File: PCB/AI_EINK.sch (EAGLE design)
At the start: 188 parts, among them IC3 WM8960, J1 BM04B-GHS-TBT(LF)(SN)(N), J2 C393939, J3 524372471, Q1 SI1308EDL-T1-GE3, Q3 NMOS_C7465427, T1 MMUN2133LT1G, U1 TPS61092RSAR, U10 AP2112-3.3K, U11 AP2112-3.3K, U12 SPU0410LR5H-QB, U2 MC74VHC1G14DFT1G, U3 BQ27441DRZR-G1A, U4 BQ24075, U5 TLV74328, U6 TLV74315, U7 TLV74318PDBVRDBV0005A_L, U8 ST25DV64K-IER6S3SOIC_IER6S3_S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, U9 EMC2301-1-ACZL-TRMSOP8_MC_MCH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, Y1 ABM8-272-T3

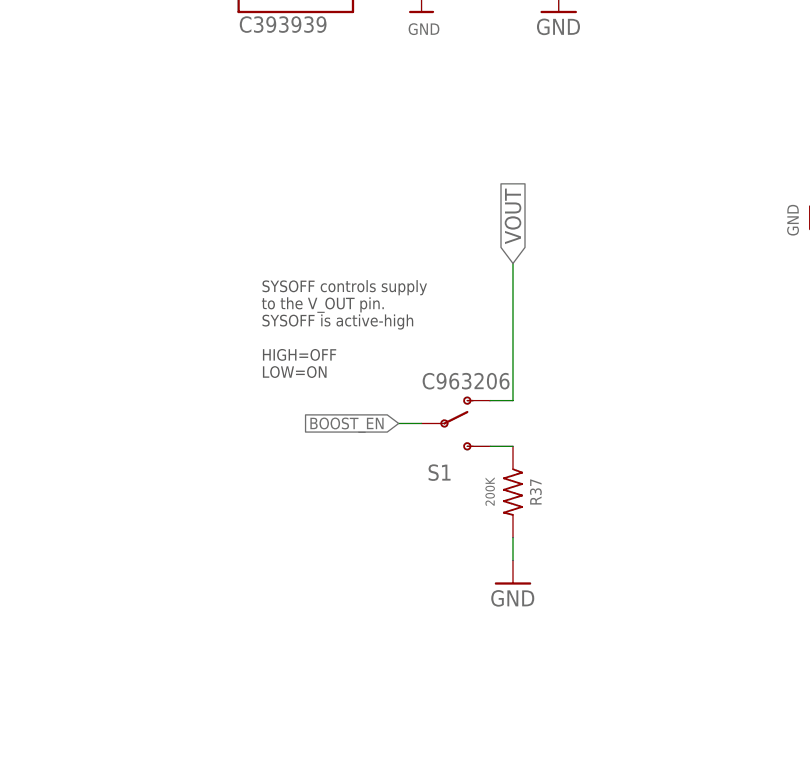
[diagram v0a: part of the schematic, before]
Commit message: kevin commit
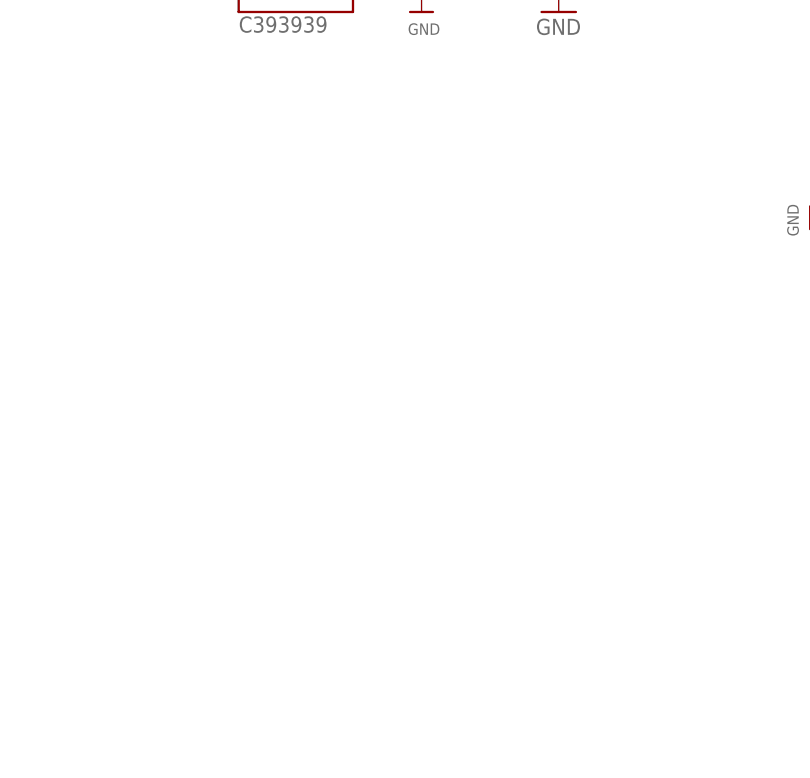
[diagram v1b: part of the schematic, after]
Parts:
- removed R37: 200K, resistor:R-US_R0603
- removed S1: C963206, SparkFun-Electromechanical:SWITCH-SPDT-SMD-A
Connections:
- removed net N$27: R37.1, S1.S
- net BOOST_EN: no longer S1.P
- net GND: no longer R37.2
- net VOUT: no longer S1.O
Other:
- note removed: "SYSOFF controls supply to the V_OUT pin. SYSOFF is active-high HIGH=OFF LOW=ON"
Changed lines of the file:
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@@
 <attribute name="PROD_ID" value="RES-13217"/>
 </part>
-<part name="GND18" library="SparkFun-Aesthetics" deviceset="GND" device=""/>
-<part name="S1" library="SparkFun-Electromechanical" deviceset="SWITCH-SPDT" device="-SMD-A" value="C963206"/>
 <part name="R7" library="resistor" library_urn="urn:adsk.eagle:library:348" deviceset="R-US_" device="R0603" package3d_urn="urn:adsk.eagle:package:23555/3" value="1.1k">
 <attribute name="PROD_ID" value="RES-10447"/>
@@
 <part name="GND35" library="SparkFun-Aesthetics" deviceset="GND" device=""/>
 <part name="R36" library="resistor" library_urn="urn:adsk.eagle:library:348" deviceset="R-US_" device="R0603" package3d_urn="urn:adsk.eagle:package:23555/3" value="200K"/>
-<part name="R37" library="resistor" library_urn="urn:adsk.eagle:library:348" deviceset="R-US_" device="R0603" package3d_urn="urn:adsk.eagle:package:23555/3" value="200K"/>
 <part name="R28" library="resistor" library_urn="urn:adsk.eagle:library:348" deviceset="R-US_" device="R0603" package3d_urn="urn:adsk.eagle:package:23555/3" value="10k"/>
 <part name="GND28" library="supply1" library_urn="urn:adsk.eagle:library:371" deviceset="GND" device=""/>
@@
      (Good IN supply)
   - Open (LED disconnected)</text>
-<text x="637.54" y="180.34" size="1.27" layer="97" font="vector">SYSOFF controls supply
-to the V_OUT pin.
-SYSOFF is active-high
-HIGH=OFF
-LOW=ON</text>
 <text x="492.76" y="106.68" size="2.54" layer="94" font="vector" align="top-left">EINK HiGH VOLTAGE MODULE</text>
 <text x="505.46" y="294.64" size="2.54" layer="94" font="vector" align="top-left">5V BOOST</text>
@@
 <attribute name="PROD_ID" x="307.34" y="226.06" size="1.524" layer="96" rot="R270" align="top-left" display="off"/>
 </instance>
-<instance part="GND18" gate="1" x="665.48" y="157.48" smashed="yes">
-<attribute name="VALUE" x="662.94" y="154.94" size="1.778" layer="96"/>
-</instance>
-<instance part="S1" gate="1" x="657.86" y="175.26" smashed="yes">
-<attribute name="NAME" x="655.955" y="168.91" size="1.778" layer="95"/>
-<attribute name="VALUE" x="655.32" y="179.07" size="1.778" layer="96"/>
-</instance>
 <instance part="R7" gate="G$1" x="322.58" y="223.52" smashed="yes" rot="R270">
 <attribute name="NAME" x="324.0786" y="227.33" size="1.778" layer="95" font="vector" rot="R270"/>
@@
 <attribute name="VALUE" x="822.96" y="198.12" size="1.016" layer="96" font="vector" ratio="15" rot="R270" align="center"/>
 </instance>
-<instance part="R37" gate="G$1" x="665.48" y="167.64" smashed="yes" rot="R270">
-<attribute name="NAME" x="668.02" y="167.64" size="1.27" layer="95" font="vector" rot="R270" align="center"/>
-<attribute name="VALUE" x="662.94" y="167.64" size="1.016" layer="96" font="vector" ratio="15" rot="R270" align="center"/>
-</instance>
 <instance part="R28" gate="G$1" x="690.88" y="76.2" smashed="yes">
 <attribute name="NAME" x="687.07" y="77.6986" size="1.778" layer="95"/>
@@
 </segment>
 <segment>
-<pinref part="GND18" gate="1" pin="GND"/>
-<pinref part="R37" gate="G$1" pin="2"/>
-<wire x1="665.48" y1="160.02" x2="665.48" y2="162.56" width="0.1524" layer="91"/>
-</segment>
-<segment>
 <pinref part="R28" gate="G$1" pin="1"/>
 <wire x1="685.8" y1="76.2" x2="680.72" y2="76.2" width="0.1524" layer="91"/>
@@
 <net name="BOOST_EN" class="0">
 <segment>
-<wire x1="655.32" y1="175.26" x2="652.78" y2="175.26" width="0.1524" layer="91"/>
-<label x="652.78" y="175.26" size="1.27" layer="95" font="vector" rot="R180" xref="yes"/>
-<pinref part="S1" gate="1" pin="P"/>
-</segment>
-<segment>
 <pinref part="R13" gate="G$1" pin="1"/>
 <wire x1="533.4" y1="274.32" x2="533.4" y2="276.86" width="0.1524" layer="91"/>
@@
 <pinref part="R36" gate="G$1" pin="1"/>
 </segment>
-<segment>
-<label x="665.48" y="193.04" size="1.778" layer="95" rot="R90" xref="yes"/>
-<wire x1="662.94" y1="177.8" x2="665.48" y2="177.8" width="0.1524" layer="91"/>
-<pinref part="S1" gate="1" pin="O"/>
-<wire x1="665.48" y1="177.8" x2="665.48" y2="193.04" width="0.1524" layer="91"/>
-</segment>
 </net>
 <net name="N$7" class="0">
@@
 </segment>
 </net>
-<net name="N$27" class="0">
-<segment>
-<pinref part="R37" gate="G$1" pin="1"/>
-<pinref part="S1" gate="1" pin="S"/>
-<wire x1="665.48" y1="172.72" x2="662.94" y2="172.72" width="0.1524" layer="91"/>
-</segment>
-</net>

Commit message: PCB V3
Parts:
- removed ANT1: NFC_ANTENNA_25X15, microbuilder:NFC_ANTENNA_25X15
- removed C25, C30: 1.0uF, Capacitor:C_CHIP-0603(1608-METRIC)
- removed C27, C70, C78, C81: 0.1uF, Capacitor:C_CHIP-0603(1608-METRIC)
- removed C28, C29, C31, C32, C33, C34, C35, C36, C37, C38, C39, C41, C51: 10uF, Capacitor:C_CHIP-0603(1608-METRIC)
- removed FB10, FB9: 120o, microbuilder:FERRITE-0805NO
- removed FL3, FL4, FL5: BLM18HE152SN1D, BLM18HE152SN1D:BLM18HE152SN1D
- removed GND25, RPIBOOT3: DNP, SparkFun-Connectors:TEST-POINT3
- removed OSC1: 24MHz 3.3V Oscillator, microbuilder:OSCILLATOR3.2X2.5
- removed OV5674: DF30FC-24DS-0.4V(82)CONN_DF30FC-24DS-0.4V(82)_HIR, 2024-03-07_05-07-01_Library:DF30FC-24DS-0.4V(82)CONN_DF30FC-24DS-0.4V(82)_HIR
- removed SJ2, SJ3: DNP, SparkFun-Passives:JUMPER-PAD-3-2OF3_NC_BY_TRACE_SMALL
- removed SPI_FLASH_SAM: W25Q128JVBIQTFBGA_128JVBIQ_WIN, 2024-03-10_02-04-46_Library:W25Q128JVBIQTFBGA_128JVBIQ_WIN
- removed U$10, U$11, U$94, U$95: MOUNTINGHOLE2.5, microbuilder:MOUNTINGHOLE2.5
- removed U7: TLV74318PDBVRDBV0005A_L, 2024-03-10_03-34-55_Library:TLV74318PDBVRDBV0005A_L
- added CAMERA: 524372271CON_524372271_MOL, 2024-03-29_02-21-27_Library:524372271CON_524372271_MOL
- added FB1, FB4: FERRITE_BEAD, Filter:FBCHIP-0603(1608-METRIC)
- added JOY_STICK: BM04B-GHS-TBT(LF)(SN)(N), BM04B-GHS-TBT_LF__SN__N_:BM04B-GHS-TBT(LF)(SN)(N)
- added M.2KEYM(NGFF): 1-2199119-5, 1-2199119-5:1-2199119-5
- added Q2: NMOS_C7465427, Transistor:NMOSFETSOT23-GSD
- added R19: 5.1K, Resistor:R-US_CHIP-0402(1005-METRIC)
- added R21: 5.1k, Resistor:R-US_CHIP-0402(1005-METRIC)
- added R25, R26: 4.7K, Resistor:R-US_CHIP-0402(1005-METRIC)
- added U13: TPD4EUSB30DQARDQA10, 2024-03-29_01-35-38_Library:TPD4EUSB30DQARDQA10
- C1, C10, C11, C12, C13, C14, C15, C16, C17, C19, C2, C20, C21, C22, C23, C26, C3, C4, C40, C43, C44, C45, C46, C47, C48, C49, C5, C50, C52, C53, C54, C57, C58, C59, C60, C61, C62, C63, C64, C65, C66, C67, C68, C69, C7, C71, C72, C73, C74, C75, C76, C77, C79, C8, C80, C82, C83, C9: device Capacitor:C_CHIP-0603(1608-METRIC) -> Capacitor:C_CHIP-0402(1005-METRIC)
- C24: value 10uF -> 0.1uF; device Capacitor:C_CHIP-0603(1608-METRIC) -> Capacitor:C_CHIP-0402(1005-METRIC)
- FB2, FB5: value Ferrite -> FERRITE_BEAD; device microbuilder:FERRITE0805 -> Filter:FBCHIP-0603(1608-METRIC)
- FB3: value Ferrite -> FERRITE_BEAD; device microbuilder:FERRITE-0805NO -> Filter:FBCHIP-0603(1608-METRIC)
- R1, R10, R11, R13, R14, R15, R16, R17, R18, R2, R20, R22, R23, R24, R28, R29, R3, R30, R31, R32, R33, R34, R35, R36, R4, R5, R6, R7, R8, R9: device resistor:R-US_R0603 -> Resistor:R-US_CHIP-0402(1005-METRIC)
- U5: value TLV74328 -> MC74VHC1G14DFT1G; device adafruit_power:VREG_SOT23-5 -> MC74VHC1G14DFT1G:MC74VHC1G14DFT1G; JLC_ROTATION 0 -> (none)
- U6: value TLV74315 -> W25Q128JVSIQSOIC_128JVSIQ_WIN-L; device adafruit_power:VREG_SOT23-5 -> 2024-03-29_04-43-21_Library:W25Q128JVSIQSOIC_128JVSIQ_WIN-L; JLC_ROTATION 0 -> (none)
- U8: value ST25DV64K-IER6S3SOIC_IER6S3_STM -> MC74VHC1G14DFT1G; device 2024-03-10_23-40-44_Library:ST25DV64K-IER6S3SOIC_IER6S3_STM -> MC74VHC1G14DFT1G:MC74VHC1G14DFT1G
- renumbered J3 to EINK_524352471
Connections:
- removed net 1.5V: C30.1, C34.1, C35.1, FL3.1, U6.OUT
- removed net 1.8V: C25.1, C28.1, C29.1, FL4.1, RPIBOOT3.1, SJ2.3, SJ3.1, U7.OUT
- removed net 2.8V: C24.1, C31.1, FL5.1, U5.OUT
- removed net AF_EN: OV5674.18
- removed net GPO: U8.GPO
- removed net N$10: FL4.2, OV5674.15
- removed net N$13: FL3.2, OV5674.13, OV5674.14
- removed net N$20: RPI-CM1G$1.GPIO16
- removed net N$22: RPI-CM1G$1.GPIO25
- removed net N$28: RPI-CM1G$1.GPIO14
- removed net N$32: ANT1.1, U8.AC1
- removed net PWDN: OV5674.19, SJ3.2
- removed net RESET: OV5674.22, SJ2.2
- removed net RFC_MCLK: OSC1.OUT, OV5674.11
- removed net SAM_GPIO0: C2040.GPIO0
- removed net SAM_GPIO10: C2040.GPIO10
- removed net SAM_GPIO11: C2040.GPIO11
- removed net SAM_GPIO12: C2040.GPIO12
- removed net SAM_GPIO13: C2040.GPIO13
- removed net SAM_GPIO14: C2040.GPIO14
- removed net SAM_GPIO15: C2040.GPIO15
- removed net SAM_GPIO23: C2040.GPIO23
- removed net SAM_GPIO24: C2040.GPIO24
- removed net SAM_GPIO9: C2040.GPIO9
- removed net SCL: IC3.SCL, OV5674.23, R18.1, RPI-CM1G$1.GPIO3, U3.SCL, U8.SCL, U9.SMCLK
- removed net SDA: IC3.SDA, OV5674.24, R15.1, RPI-CM1G$1.GPIO2, U3.SDA, U8.SDA, U9.SMDATA
- removed net STROBE: OV5674.20
- removed net SYS_POW_SAM: C2040.GPIO21, Q3.G
- removed net VEH: U8.V_EH
- new net 3V3_EINK: C17.1, C9.1, EINK_524352471.10, EINK_524352471.9, L2.1, Q2.S
- new net CAM1_C_N: CAMERA.8, RPI-CM1G$2.CAM1_C_N
- new net CAM1_C_P: CAMERA.9, RPI-CM1G$2.CAM1_C_P
- new net CAM1_D0_N: CAMERA.2, RPI-CM1G$2.CAM1_D0_N
- new net CAM1_D0_P: CAMERA.3, RPI-CM1G$2.CAM1_D0_P
- new net CAM1_D1_N: CAMERA.5, RPI-CM1G$2.CAM1_D1_N
- new net CAM1_D1_P: CAMERA.6, RPI-CM1G$2.CAM1_D1_P
- new net CAM1_D2_N: CAMERA.11, RPI-CM1G$2.CAM1_D2_N
- new net CAM1_D2_P: CAMERA.12, RPI-CM1G$2.CAM1_D2_P
- new net CAM1_D3_N: CAMERA.14, RPI-CM1G$2.CAM1_D3_N
- new net CAM1_D3_P: CAMERA.15, RPI-CM1G$2.CAM1_D3_P
- new net DSI0_C_N: RPI-CM1G$2.DSI0_C_N
- new net DSI0_C_P: RPI-CM1G$2.DSI0_C_P
- new net DSI0_D0_N: RPI-CM1G$2.DSI0_D0_N
- new net DSI0_D0_P: RPI-CM1G$2.DSI0_D0_P
- new net DSI0_D1_N: RPI-CM1G$2.DSI0_D1_N
- new net DSI0_D1_P: RPI-CM1G$2.DSI0_D1_P
- new net DSI1_C_N: RPI-CM1G$2.DSI1_C_N
- new net DSI1_C_P: RPI-CM1G$2.DSI1_C_P
- new net DSI1_D0_N: RPI-CM1G$2.DSI1_D0_N
- new net DSI1_D0_P: RPI-CM1G$2.DSI1_D0_P
- new net DSI1_D1_N: RPI-CM1G$2.DSI1_D1_N
- new net DSI1_D1_P: RPI-CM1G$2.DSI1_D1_P
- new net DSI1_D2_N: RPI-CM1G$2.DSI1_D2_N
- new net DSI1_D2_P: RPI-CM1G$2.DSI1_D2_P
- new net DSI1_D3_N: RPI-CM1G$2.DSI1_D3_N
- new net DSI1_D3_P: RPI-CM1G$2.DSI1_D3_P
- new net EXT_VCC_PCIE: M.2KEYM(NGFF).P12, M.2KEYM(NGFF).P14, M.2KEYM(NGFF).P16, M.2KEYM(NGFF).P18, M.2KEYM(NGFF).P2, M.2KEYM(NGFF).P4, M.2KEYM(NGFF).P70, M.2KEYM(NGFF).P72, M.2KEYM(NGFF).P74
- new net HDMI0_CEC: RPI-CM1G$2.HDMI0_CEC
- new net HDMI0_CLK_N: RPI-CM1G$2.HDMI0_CLK_N
- new net HDMI0_CLK_P: RPI-CM1G$2.HDMI0_CLK_P
- new net HDMI0_HOTPLUG: RPI-CM1G$2.HDMI0_HOTPLUG
- new net HDMI0_SCL: RPI-CM1G$2.HDMI0_SCL
- new net HDMI0_SDA: RPI-CM1G$2.HDMI0_SDA
- new net HDMI0_TX0_N: RPI-CM1G$2.HDMI0_TX0_N
- new net HDMI0_TX0_P: RPI-CM1G$2.HDMI0_TX0_P
- new net HDMI0_TX1_N: RPI-CM1G$2.HDMI0_TX1_N
- new net HDMI0_TX1_P: RPI-CM1G$2.HDMI0_TX1_P
- new net HDMI0_TX2_N: RPI-CM1G$2.HDMI0_TX2_N
- new net HDMI0_TX2_P: RPI-CM1G$2.HDMI0_TX2_P
- new net HDMI1_CEC: RPI-CM1G$2.HDMI1_CEC
- new net HDMI1_CLK_N: RPI-CM1G$2.HDMI1_CLK_N
- new net HDMI1_CLK_P: RPI-CM1G$2.HDMI1_CLK_P
- new net HDMI1_HOTPLUG: RPI-CM1G$2.HDMI1_HOTPLUG
- new net HDMI1_SCL: RPI-CM1G$2.HDMI1_SCL
- new net HDMI1_SDA: RPI-CM1G$2.HDMI1_SDA
- new net HDMI1_TX0_N: RPI-CM1G$2.HDMI1_TX0_N
- new net HDMI1_TX0_P: RPI-CM1G$2.HDMI1_TX0_P
- new net HDMI1_TX1_N: RPI-CM1G$2.HDMI1_TX1_N
- new net HDMI1_TX1_P: RPI-CM1G$2.HDMI1_TX1_P
- new net HDMI1_TX2_N: RPI-CM1G$2.HDMI1_TX2_N
- new net HDMI1_TX2_P: RPI-CM1G$2.HDMI1_TX2_P
- new net N$27: J2.CC2, R21.2
- new net N$30: J2.CC1, R19.2
- new net PCIE_!RST: M.2KEYM(NGFF).P50, RPI-CM1G$2.PCIE_!RST
- new net PCIE_CLK_!REQ: M.2KEYM(NGFF).P52, RPI-CM1G$2.PCIE_CLK_!REQ
- new net PCIE_CLK_N: M.2KEYM(NGFF).P53, RPI-CM1G$2.PCIE_CLK_N
- new net PCIE_CLK_P: M.2KEYM(NGFF).P55, RPI-CM1G$2.PCIE_CLK_P
- new net PCIE_RX_N: M.2KEYM(NGFF).P41, RPI-CM1G$2.PCIE_RX_N
- new net PCIE_RX_P: M.2KEYM(NGFF).P43, RPI-CM1G$2.PCIE_RX_P
- new net PCIE_TX_N: M.2KEYM(NGFF).P47, RPI-CM1G$2.PCIE_TX_N
- new net PCIE_TX_P: M.2KEYM(NGFF).P49, RPI-CM1G$2.PCIE_TX_P
- new net RESERVED@104: RPI-CM1G$2.RESERVED@104
- new net RESERVED@106: RPI-CM1G$2.RESERVED@106
- new net SAM_EINK_ON: C2040.GPIO9, U5.IN_A
- new net SAM_INTERUPT: C2040.GPIO0, RPI-CM1G$1.GPIO22
- new net SAM_SCL: C2040.GPIO23, JOY_STICK.3, R26.1, U3.SCL
- new net SAM_SDA: C2040.GPIO24, JOY_STICK.2, R25.1, U3.SDA
- new net SCL0: CAMERA.20, RPI-CM1G$1.SCL0
- new net SCL1: IC3.SCL, R18.1, RPI-CM1G$1.GPIO3, U9.SMCLK
- new net SDA0: CAMERA.21, RPI-CM1G$1.SDA0
- new net SDA1: IC3.SDA, R15.1, RPI-CM1G$1.GPIO2, U9.SMDATA
- new net SYS_PI_ON: C2040.GPIO21, U8.IN_A
- new net USB_OTG_ID: RPI-CM1G$2.USB_OTG_ID
- new net VDAC_COMP: RPI-CM1G$2.VDAC_COMP
- net 3.3V: now also CAMERA.22, Q2.D; no longer C17.1, C26.1, C27.1, C32.1, C33.1, C36.1, C37.1, C38.1, C39.1, C9.1, EINK_524352471.10, EINK_524352471.9, L2.1, OSC1.INH, OSC1.VCC, U5.EN, U5.IN, U6.EN, U6.IN, U7.EN, U7.IN, U8.VCC
- net AGND: now also FB5.2; no longer FB5.P$1
- net AVDD: now also FB1.2; no longer FB2.P$1
- net CAM0_C_N: no longer OV5674.8
- net CAM0_C_P: no longer OV5674.9
- net CAM0_D0_N: no longer OV5674.2
- net CAM0_D0_P: no longer OV5674.3
- net CAM0_D1_N: no longer OV5674.5
- net CAM0_D1_P: no longer OV5674.6
- net CAM_GPIO: now also CAMERA.17
- net EINK_BUSY: now also C2040.GPIO10
- net EINK_CS: now also C2040.GPIO13
- net EINK_D/C: now also C2040.GPIO12
- net EINK_RESET: now also C2040.GPIO11
- net GND: now also C24.1, CAMERA.1, CAMERA.10, CAMERA.13, CAMERA.16, CAMERA.19, CAMERA.4, CAMERA.7, FB5.1, JOY_STICK.4, M.2KEYM(NGFF).P1, M.2KEYM(NGFF).P15, M.2KEYM(NGFF).P21, M.2KEYM(NGFF).P27, M.2KEYM(NGFF).P3, M.2KEYM(NGFF).P33, M.2KEYM(NGFF).P39, M.2KEYM(NGFF).P45, M.2KEYM(NGFF).P51, M.2KEYM(NGFF).P57, M.2KEYM(NGFF).P71, M.2KEYM(NGFF).P73, M.2KEYM(NGFF).P75, M.2KEYM(NGFF).P9, M.2KEYM(NGFF).SHIELD, R19.1, R21.1, U13.GND, U8.GND; no longer C24.2, C25.2, C27.2, C28.2, C29.2, C30.2, C31.2, C32.2, C33.2, C34.2, C35.2, C36.2, C37.2, C38.2, C39.2, C41.2, C51.2, C70.2, C78.2, C81.2, FB5.P$2, GND25.1, OSC1.GND, OV5674.1, OV5674.10, OV5674.12, OV5674.21, OV5674.4, OV5674.7, SJ2.1, SJ3.3, SPI_FLASH_SAM.GND, U7.GND, U8.VSS
- net LEFT_N: now also FB3.2; no longer FB10.P$2
- net LEFT_P: now also FB2.2; no longer FB9.P$2
- net N$16: now also Q3.G, U8.OUT_~Y; no longer ANT1.2, U8.AC0
- net N$29: now also FB4.1; no longer FB3.P$1
- net N$36: now also FB4.2; no longer FB3.P$2
- net N$40: now also FB2.1; no longer FB9.P$1
- net N$41: now also FB3.1; no longer FB10.P$1
- net N$8: now also Q2.G, U5.OUT_~Y; no longer FL5.2, OV5674.16, OV5674.17
- net OUT: now also FB1.1; no longer FB2.P$2
- net SAM_1V1: no longer C78.1
- net SAM_3V3: now also C24.2, JOY_STICK.1, R25.2, R26.2, U5.VCC, U6.VCC, U8.VCC; no longer C70.1, C81.1, SPI_FLASH_SAM.VCC
- net SAM_QSPI_SCLK: now also U6.CLK; no longer SPI_FLASH_SAM.CLK
- net SAM_QSPI_SCN: now also U6./CS; no longer SPI_FLASH_SAM./CS
- net SAM_QSPI_SD0: now also U6.DI_(IO0); no longer SPI_FLASH_SAM.DI_(IO0)
- net SAM_QSPI_SD1: now also U6.DO_(IO1); no longer SPI_FLASH_SAM.DO_(IO1)
- net SAM_QSPI_SD2: now also U6./WP_(IO2); no longer SPI_FLASH_SAM./WP_(IO2)
- net SAM_QSPI_SD3: now also U6./HOLD_OR_/RESET_(IO3); no longer SPI_FLASH_SAM./HOLD_(IO3)
- net SPI_CLK: now also C2040.GPIO14
- net SPI_MOSI: now also C2040.GPIO15
- net USB_N: now also U13.D2-
- net USB_P: now also U13.D2+
- net VOUT: now also C26.1
- net V_BATT: no longer C41.1, C51.1
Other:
- moved on the sheet: C20, C24, C26, C3, C54, C57, C63, C64, C67, C68, C7, C82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
